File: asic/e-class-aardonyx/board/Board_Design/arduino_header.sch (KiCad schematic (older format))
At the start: 31 parts, among them J10 Conn_1x6_F, J11 Conn_1x6_F, J12 Conn_1x3_M, J13 Conn_1x8, J14 Conn_1x6_F, J15 Conn_1x10, J16 Conn_1x8, J7 Conn_1X4, J8 Conn_1x3_M, J9 Conn_1x8, U5 CAT24M01WI-GT3, U6 IS25LP256x-xM, U7 MCP3008, U8 LSF0108PWR, U9 LSF0108PWR

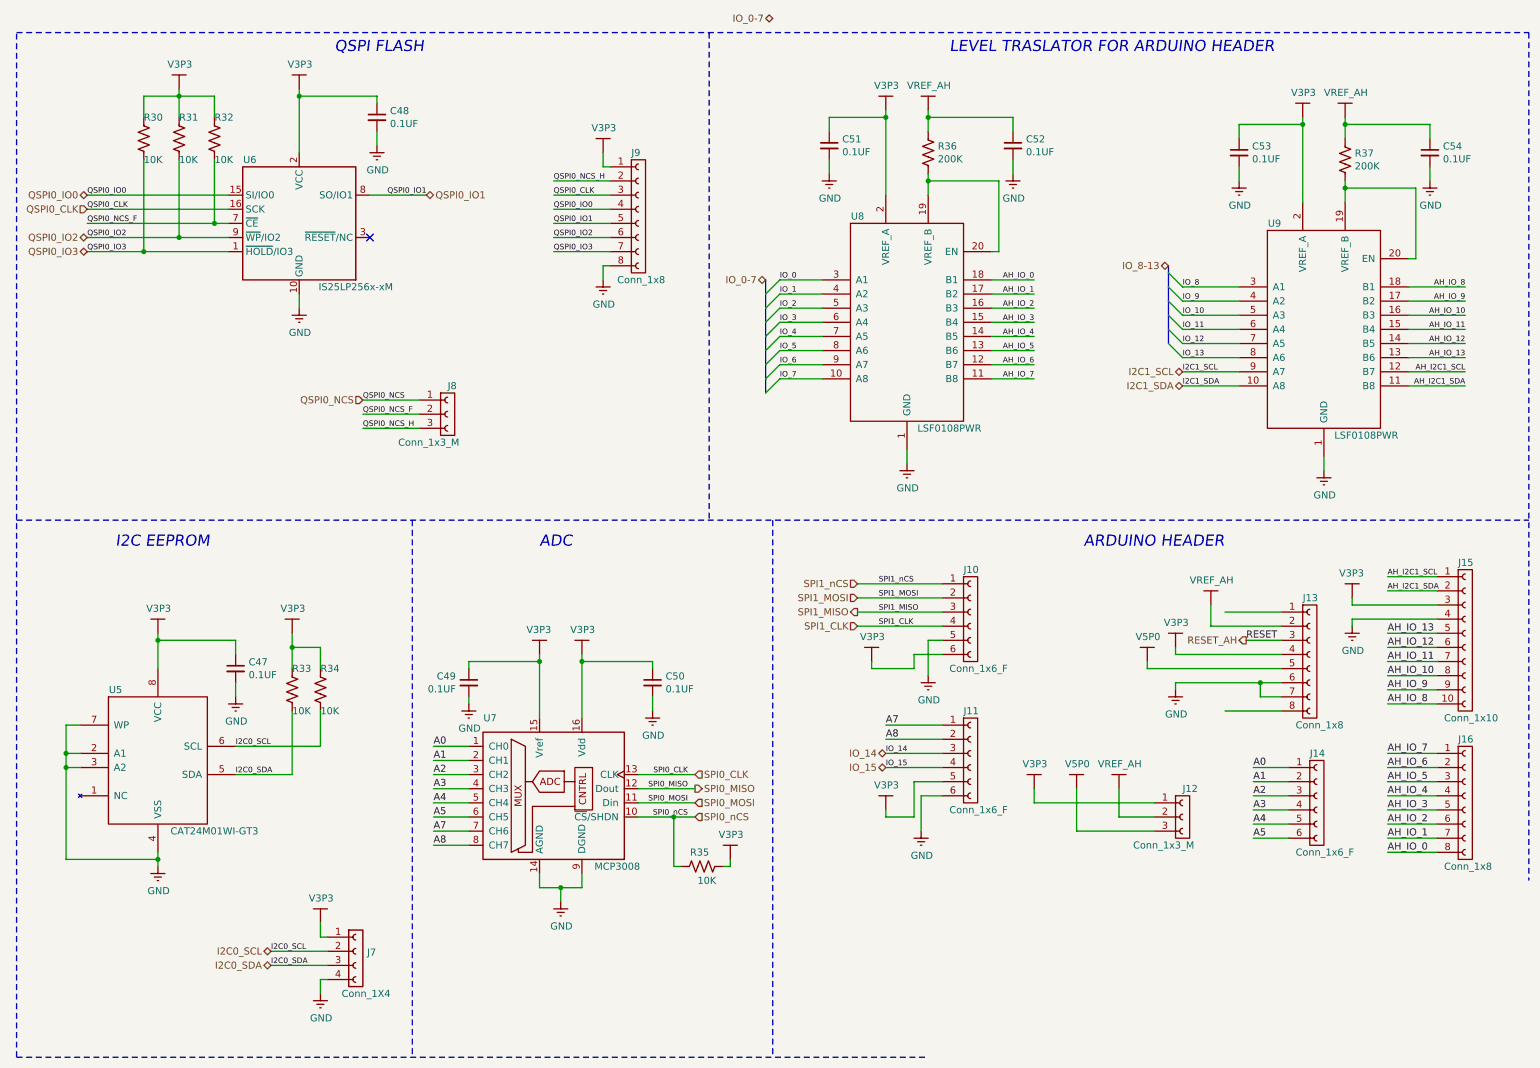
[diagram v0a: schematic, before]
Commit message: update
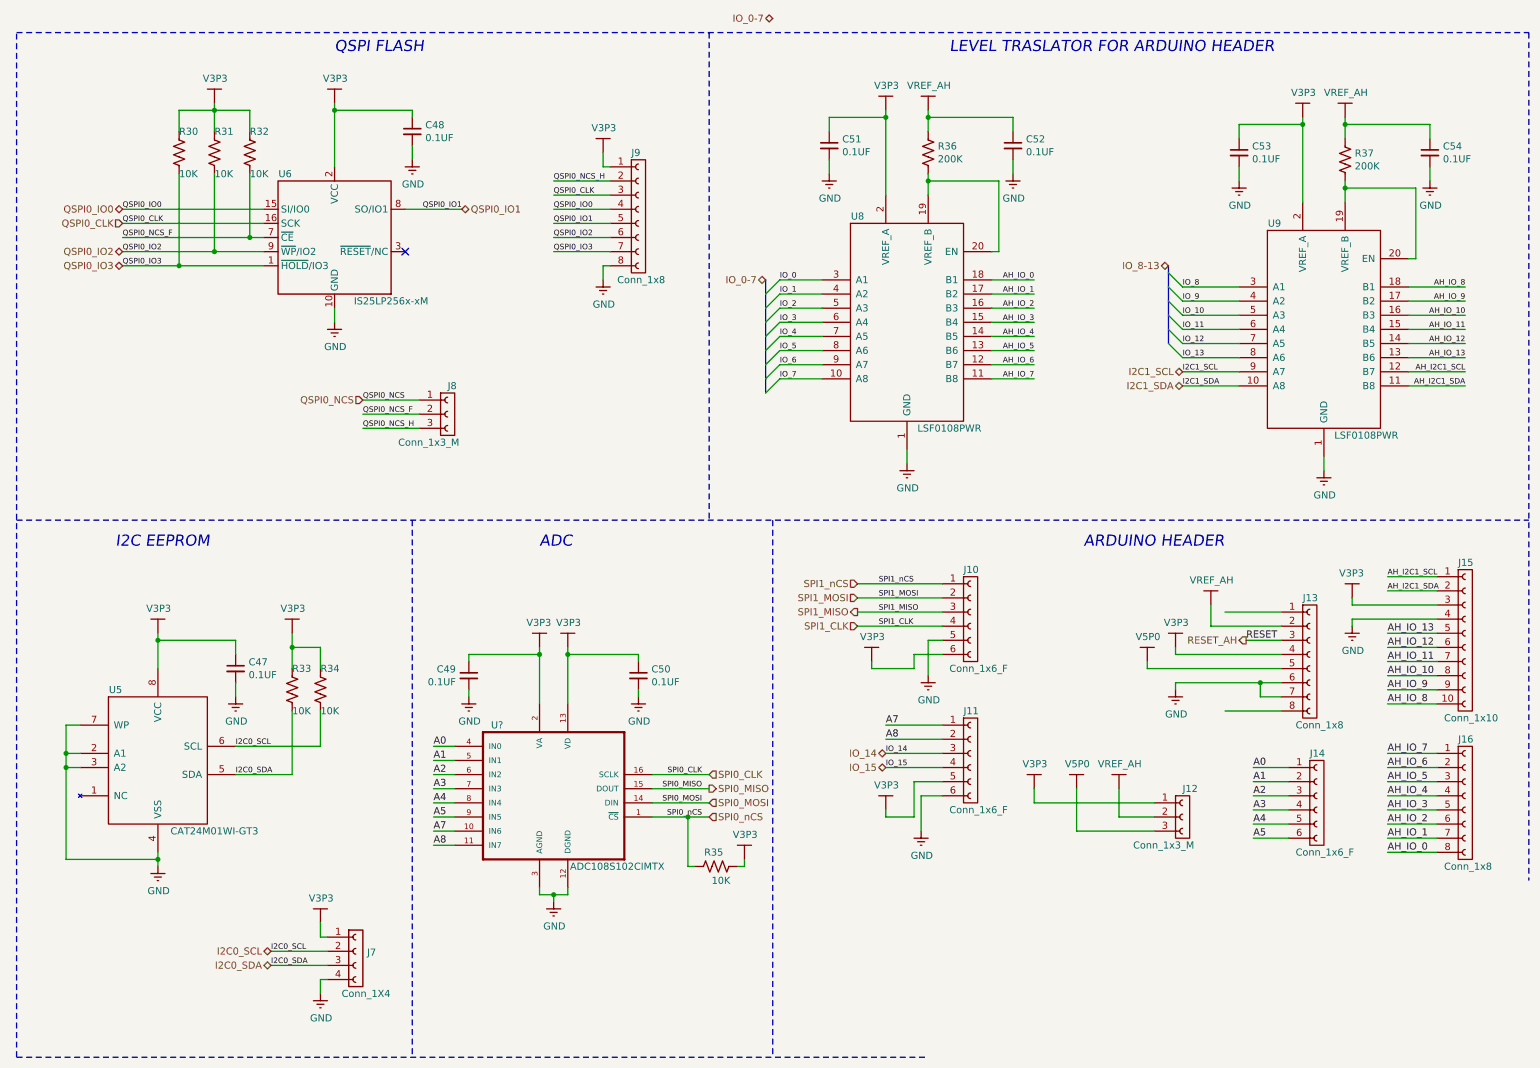
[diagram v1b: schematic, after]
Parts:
- removed U7: MCP3008, symbol aardonyx:MCP3008
- added U?: ADC108S102CIMTX, symbol aardonyx:ADC108S102CIMTX_NOPB
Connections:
- net A0: now also U?.4 (IN0)
- net A1: now also U?.5 (IN1)
- net A2: now also U?.6 (IN2)
- net A3: now also U?.7 (IN3)
- net A4: now also U?.8 (IN4)
- net A5: now also U?.9 (IN5)
- net A7: now also U?.10 (IN6)
- net A8: now also U?.11 (IN7)
- net GNDREF: now also U?.12 (DGND), U?.3 (AGND)
- net SPI0_CLK: now also U?.16 (SCLK)
- net SPI0_MISO: now also U?.15 (DOUT)
- net SPI0_MOSI: now also U?.14 (DIN)
- net SPI0_nCS: now also U?.1 (~CS)
- net at C49.1: now also U?.2 (VA)
- net at C50.1: now also U?.13 (VD)
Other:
- moved on the sheet: C48, C49, C50, R30, R31, R32, R35, U6
